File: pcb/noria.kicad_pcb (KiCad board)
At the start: 2 copper layers, 160.8 x 113.7 mm, 106 parts, among them J10 MJ-4PP-9, J2 USB_C_Receptacle_USB2.0, J3 USB_C_Receptacle_USB2.0, J4 SWD, J5 Conn_01x05, J6 Conn_01x03, J7 display, J8 Conn_01x03, J9 MJ-4PP-9, SW1 SW_PUSH, SW10 SW_PUSH, SW11 SW_PUSH, SW12 SW_PUSH, SW13 SW_PUSH, SW14 SW_PUSH, SW15 SW_PUSH, SW16 SW_PUSH, SW17 SW_PUSH, SW18 SW_PUSH, SW19 SW_PUSH, SW2 SW_PUSH, SW20 SW_PUSH, SW21 SW_PUSH, SW22 SW_PUSH, SW23 SW_PUSH, SW24 SW_PUSH, SW25 SW_PUSH, SW26 SW_PUSH, SW27 SW_PUSH, SW28 Rotary_Encoder, SW29 Rotary_Encoder, SW3 SW_PUSH, SW30 Rotary_Encoder, SW4 SW_PUSH, SW5 SW_PUSH, SW6 SW_PUSH, SW7 SW_PUSH, SW8 SW_PUSH, SW9 SW_PUSH, U1 MX25R3235FM1xx0, U2 holyiot18010, U3 holyiot18010, U4 MX25R3235FM1xx0, U5 TLV73333PDBV, U6 TLV73333PDBV

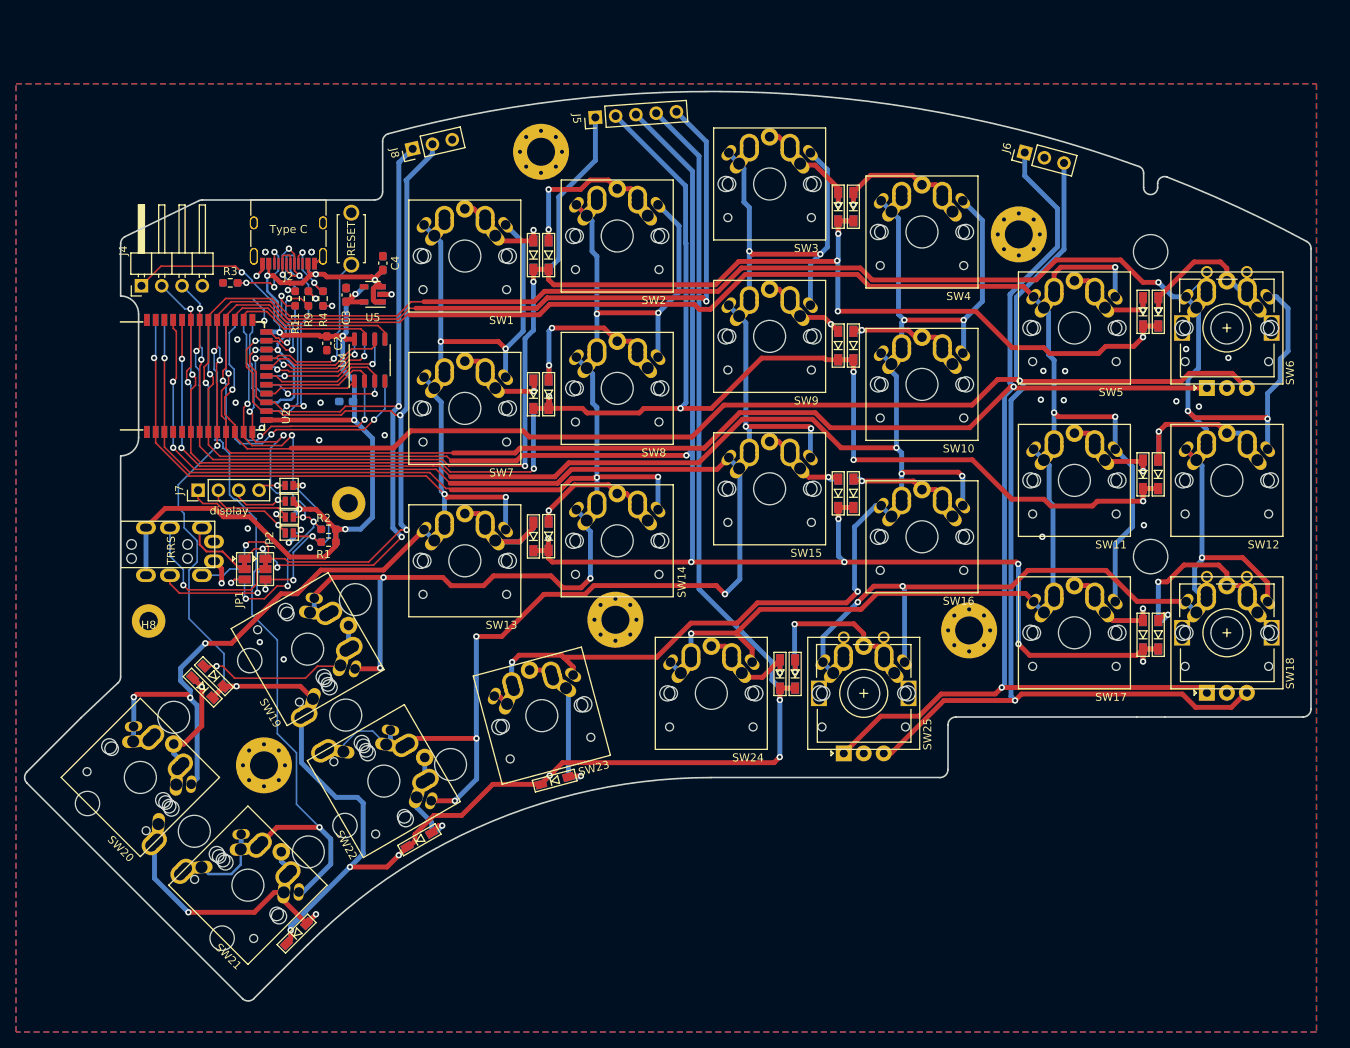
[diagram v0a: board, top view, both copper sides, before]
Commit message: Update to latest design
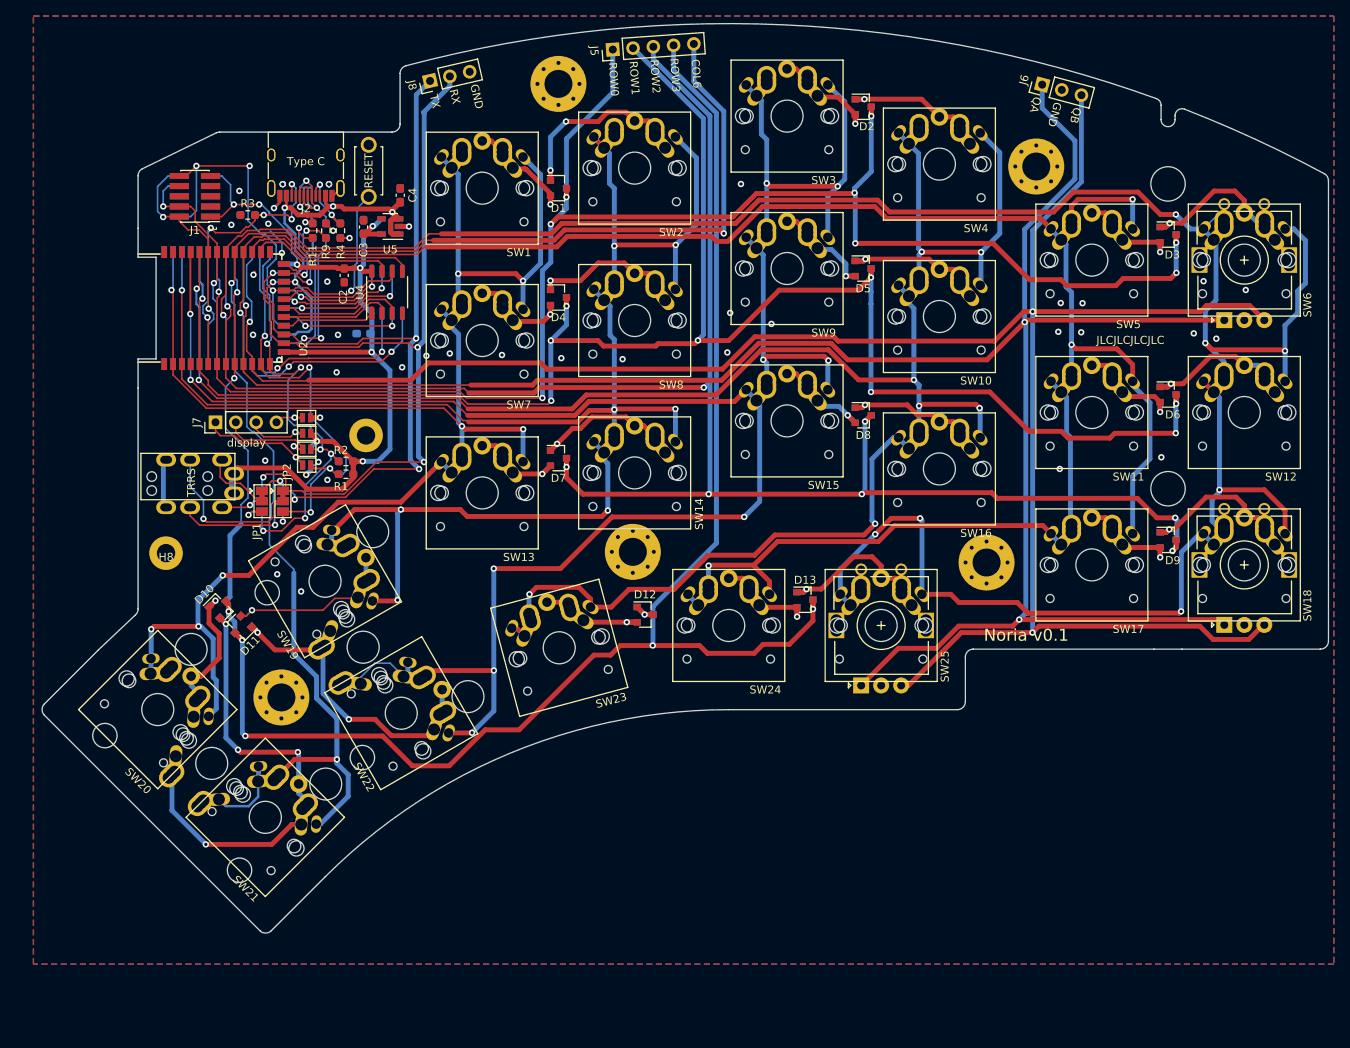
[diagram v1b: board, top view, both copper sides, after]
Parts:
- removed D14, D15, D16, D17, D18, D19, D20, D21, D22, D23, D24, D25: D, lib:D3_SMD_v2_mirror
- added J1: Conn_02x05_Odd_Even, Connector_PinHeader_1.27mm:PinHeader_2x05_P1.27mm_Vertical_SMD, F.Cu at (87.1, 52.0)
- D1, D10, D11, D13, D2, D3, D4, D5, D6, D7, D8, D9: value D -> BAS40-05; footprint lib:D3_SMD_v2_mirror -> lib:SOT-23_mirror; moved to B.Cu
- D12: value D -> BAS40-05; footprint lib:D3_SMD_v2_mirror -> lib:SOT-23_mirror
- J4: value SWD -> Conn_02x05_Odd_Even; footprint Connector_PinHeader_2.54mm:PinHeader_1x04_P2.54mm_Horizontal -> Connector_PinHeader_1.27mm:PinHeader_2x05_P1.27mm_Vertical_SMD; moved to B.Cu
- U1, U4: value MX25R3235FM1xx0 -> BY25Q32BSTIG(T)
- moved D11 114.4 mm to (92.8, 105.9), turned to 225 degrees
- moved D10 85.6 mm to (90.3, 103.3), turned to 45 degrees
- moved D12 66.5 mm to (143.4, 104.3), turned to 0 degrees
- moved D9 47.9 mm to (208.8, 95.0), turned to 0 degrees
- moved D2 43.5 mm to (170.7, 40.8), turned to 0 degrees
- moved D3 41.4 mm to (208.8, 56.8), turned to 0 degrees
- moved D8 39.4 mm to (170.7, 79.4), turned to 0 degrees
- moved D4 38.6 mm to (132.6, 64.7), turned to 0 degrees
- moved D5 35.4 mm to (170.6, 61.1), turned to 0 degrees
- moved D13 34.9 mm to (163.4, 102.5), turned to 0 degrees
- moved J4 13.0 mm to (87.1, 52.0), turned to 180 degrees
- moved D6 10.4 mm to (208.8, 76.8), turned to 0 degrees
- moved D1 8.93 mm to (132.6, 51.0), turned to 0 degrees
- moved J10 8.85 mm to (80.2, 87.1)
- moved J9 8.85 mm to (80.2, 88.8)
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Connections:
- D1 pad 1: /ROW0 -> Net-(D1-Pad1)
- D10 pad 1: /ROW1 -> Net-(D10-Pad1)
- D11 pad 1: /ROW1 -> Net-(D11-Pad1)
- D12 pad 1: /ROW1 -> /ROW3
- D13 pad 1: /ROW2 -> Net-(D13-Pad1)
- D2 pad 1: /ROW0 -> Net-(D2-Pad1)
- D3 pad 1: /ROW0 -> Net-(D3-Pad1)
- D4 pad 1: /ROW0 -> Net-(D4-Pad1)
- D5 pad 1: /ROW0 -> Net-(D5-Pad1)
- D6 pad 1: /ROW0 -> Net-(D6-Pad1)
- D7 pad 1: /ROW1 -> Net-(D7-Pad1)
- D8 pad 1: /ROW1 -> Net-(D8-Pad1)
- D9 pad 1: /ROW1 -> Net-(D9-Pad1)
- J10 pad A: GND -> +3V3
- J10 pad B: +3V3 -> GND
- J4 pad 3: /SWCLK -> GND
- J4 pad 4: GND -> /SWCLK
- J9 pad A: GND -> +3V3
- J9 pad B: +3V3 -> GND
- SW1 pad 2: Net-(D1-Pad2) -> Net-(D1-Pad1)
- SW10 pad 2: Net-(D10-Pad2) -> Net-(D5-Pad2)
- SW11 pad 2: Net-(D11-Pad2) -> Net-(D6-Pad1)
- SW12 pad 2: Net-(D12-Pad2) -> Net-(D6-Pad2)
- SW13 pad 2: Net-(D13-Pad2) -> Net-(D7-Pad1)
- SW14 pad 2: Net-(D14-Pad2) -> Net-(D7-Pad2)
- SW15 pad 2: Net-(D15-Pad2) -> Net-(D8-Pad1)
- SW16 pad 2: Net-(D16-Pad2) -> Net-(D8-Pad2)
- SW17 pad 2: Net-(D17-Pad2) -> Net-(D9-Pad1)
- SW18 pad 2: Net-(D18-Pad2) -> Net-(D9-Pad2)
- SW19 pad 2: Net-(D19-Pad2) -> Net-(D11-Pad1)
- SW2 pad 2: Net-(D2-Pad2) -> Net-(D1-Pad2)
- SW20 pad 2: Net-(D20-Pad2) -> Net-(D10-Pad2)
- SW21 pad 2: Net-(D21-Pad2) -> Net-(D10-Pad1)
- SW22 pad 2: Net-(D22-Pad2) -> Net-(D11-Pad2)
- SW23 pad 2: Net-(D23-Pad2) -> Net-(D12-Pad2)
- SW24 pad 2: Net-(D24-Pad2) -> Net-(D13-Pad1)
- SW25 pad 2: Net-(D25-Pad2) -> Net-(D13-Pad2)
- SW26 pad 2: Net-(D21-Pad2) -> Net-(D10-Pad1)
- SW27 pad 2: /ROW3 -> Net-(D11-Pad2)
- SW3 pad 2: Net-(D3-Pad2) -> Net-(D2-Pad1)
- SW4 pad 2: Net-(D4-Pad2) -> Net-(D2-Pad2)
- SW5 pad 2: Net-(D5-Pad2) -> Net-(D3-Pad1)
- SW6 pad 2: Net-(D6-Pad2) -> Net-(D3-Pad2)
- SW7 pad 2: Net-(D7-Pad2) -> Net-(D4-Pad1)
- SW8 pad 2: Net-(D8-Pad2) -> Net-(D4-Pad2)
- SW9 pad 2: Net-(D9-Pad2) -> Net-(D5-Pad1)
- U2 pad 5: (no net) -> /ROW1
- U2 pad 6: /ROW1 -> /CC1
- U3 pad 36: (no net) -> GND
- U3 pad 5: (no net) -> /ROW1
- U3 pad 6: /ROW1 -> /CC1
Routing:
- net Net-(D10-Pad1): track 0.00 -> 65.9 mm, vias 0 -> 4
- net Net-(D21-Pad2): track 44.1 -> 0.00 mm, vias 2 -> 0
- net /nReset: track 28.1 -> 63.6 mm, vias 2 -> 4
- net /ROW3: track 265.9 -> 237.1 mm, vias 9 -> 8
- net Net-(D11-Pad2): track 13.6 -> 41.6 mm, vias 1 -> 2
- net Net-(D19-Pad2): track 25.9 -> 0.00 mm, vias 1 -> 0
- net /CC1: track 12.1 -> 36.7 mm, vias 3 -> 5
- net Net-(D25-Pad2): track 24.2 -> 0.00 mm, vias 2 -> 0
- net Net-(D18-Pad2): track 24.2 -> 0.00 mm, vias 2 -> 0
- net Net-(D11-Pad1): track 0.00 -> 23.3 mm, vias 0 -> 1
- net Net-(D23-Pad2): track 20.1 -> 0.00 mm, vias 1 -> 0
- net Net-(D14-Pad2): track 19.4 -> 0.00 mm, vias 1 -> 0
- net Net-(D20-Pad2): track 18.0 -> 0.00 mm, vias 1 -> 0
- net Net-(D16-Pad2): track 16.2 -> 0.00 mm, vias 1 -> 0
- net +3V3: track 134.0 -> 118.3 mm, vias 7 -> 8
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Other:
- outline, holes or cut-outs redrawn
- board text added: "1"
- board text added: "COL6"
- board text added: "GND"
- board text added: "JLCJLCJLCJLC"
- board text added: "Noria v0.1"
- board text added: "QA"
- board text added: "QB"
- board text added: "ROW0"
- board text added: "ROW1"
- board text added: "ROW2"
- board text added: "ROW3"
- board text added: "RX"
- board text added: "TX"

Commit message: And another update
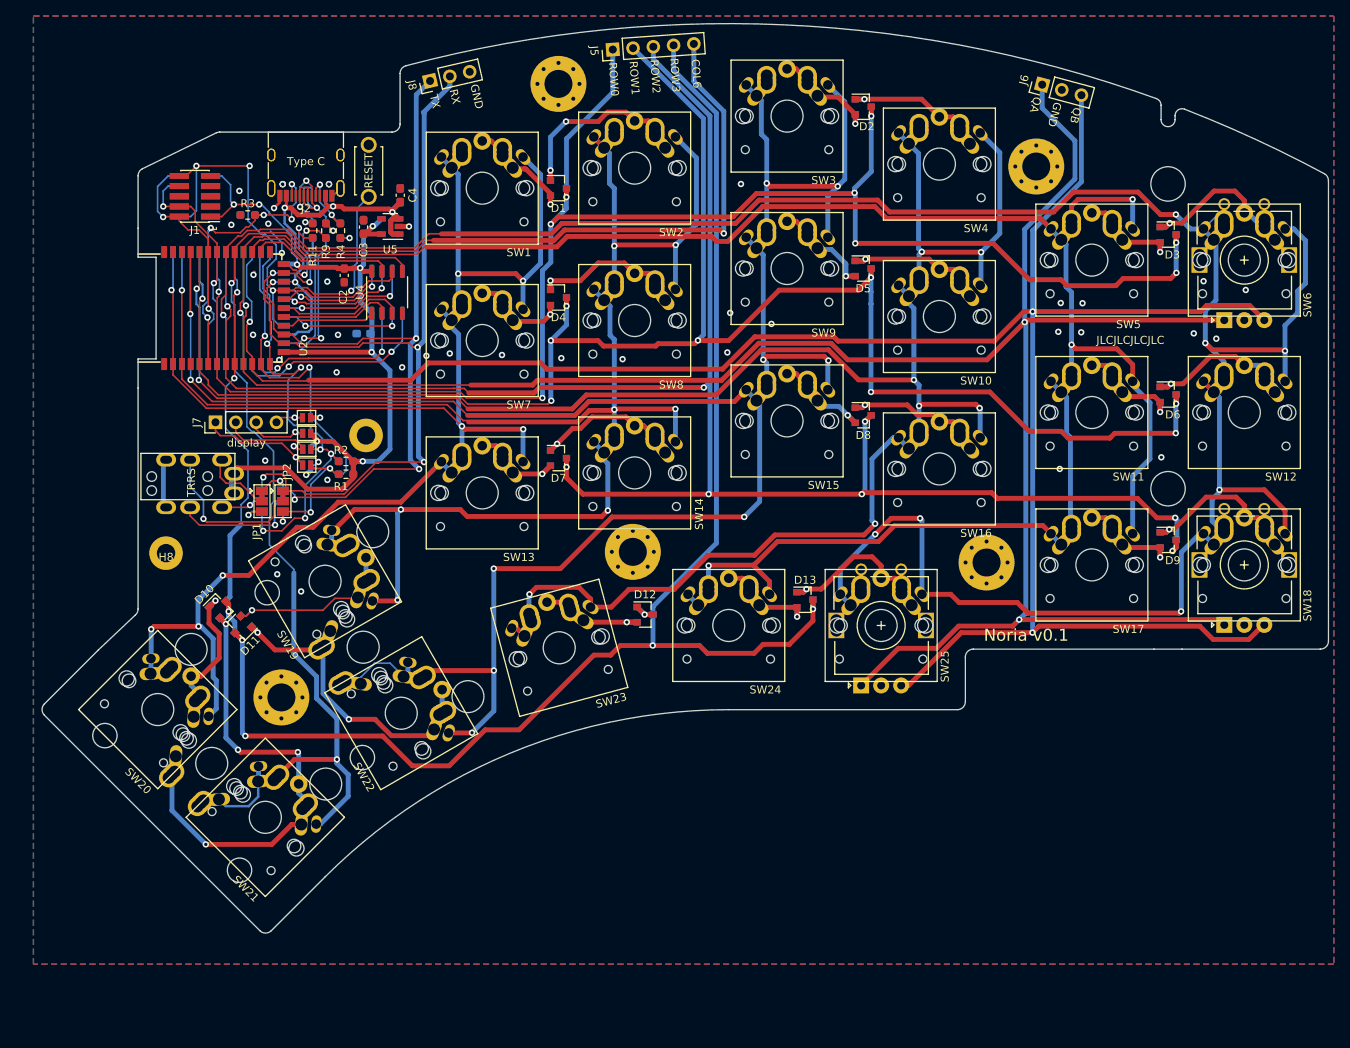
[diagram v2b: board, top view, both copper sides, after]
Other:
- net class Default removed
